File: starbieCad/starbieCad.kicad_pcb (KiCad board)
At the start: 2 copper layers, 76.3 x 68.9 mm, 7 parts, among them J1 Conn_01x04_Pin, J2 Conn_01x08_Pin, SW1 SW_Push, SW2 SW_Push, U1 DHT11, U2 XIAO-ESP32-C3-SMD

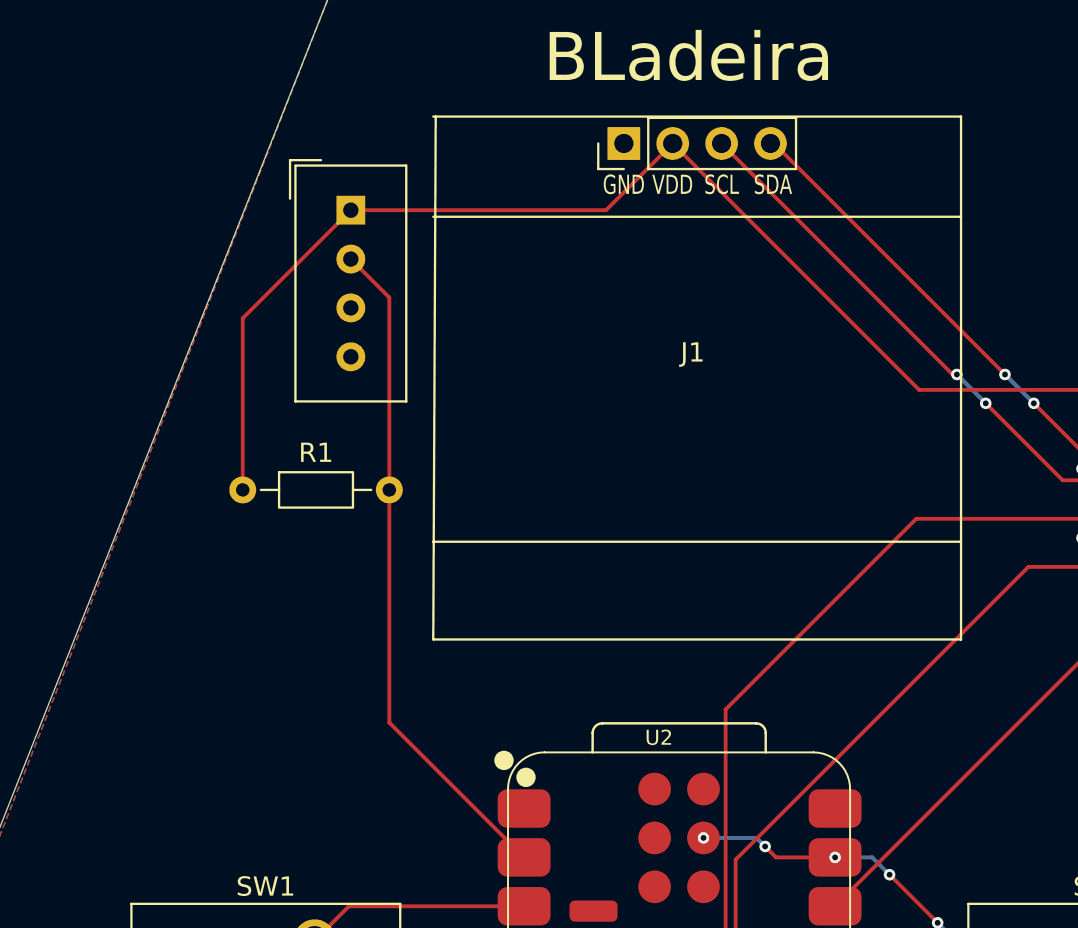
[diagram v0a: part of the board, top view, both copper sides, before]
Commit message: I added images in the starbie shape but whit a lot of struggle
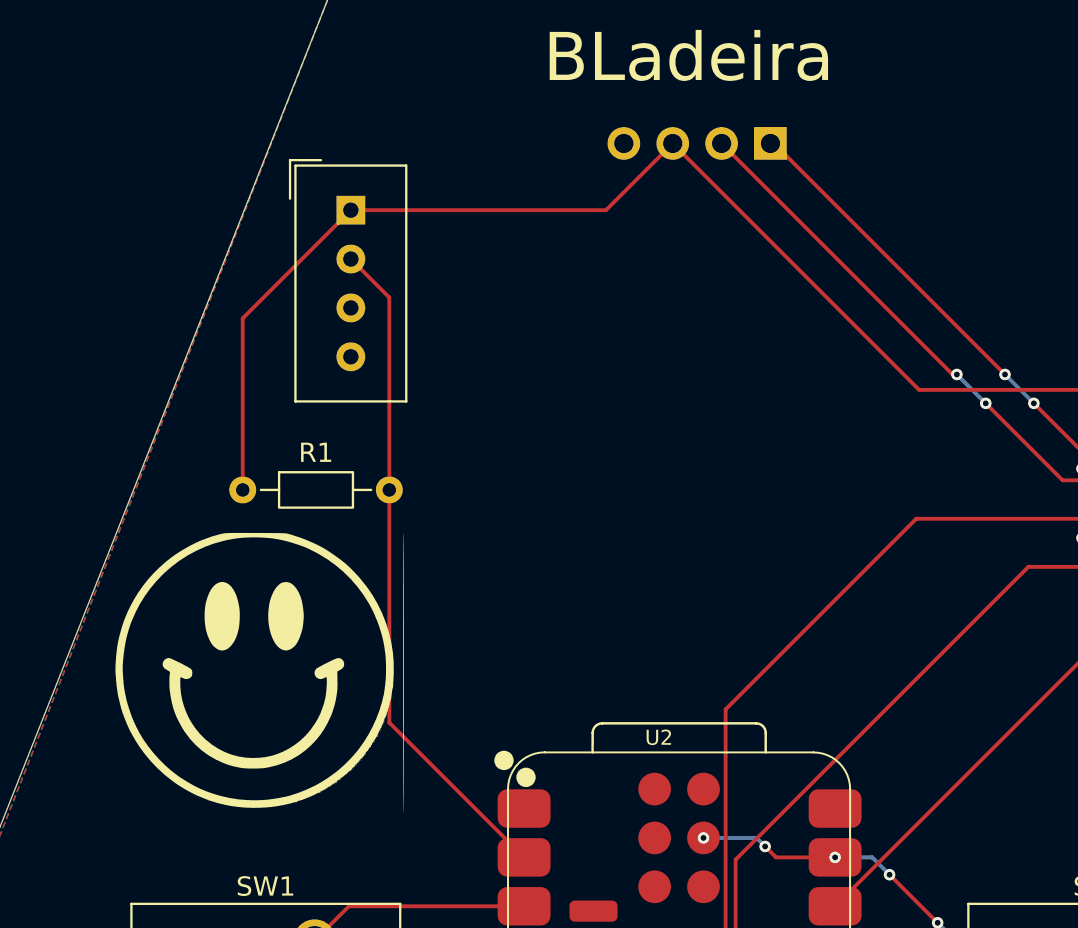
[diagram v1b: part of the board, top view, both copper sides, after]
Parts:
- added G***: LOGO, LOGO, F.Cu at (127.2, 100.0)
- added G***: LOGO, LOGO, B.Cu at (148.2, 98.0)
- J1: moved to B.Cu
- turned J1 to 180 degrees
